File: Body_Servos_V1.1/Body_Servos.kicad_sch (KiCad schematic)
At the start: 30 parts, among them J1 USB_B_Micro, J12 SERIAL_FU, J2 AUX3, J3 AUX1, J4 AUX2, J5 12OUT, J6 12VOUT, J7 5V OUT, J8 5V Out 2, SW1 SW_Push, U1 ESP32-WROOM-32D_16MB_, U2 CJ2301_S1, U3 ME6211C33M5G, U4 CH340C, U5 UMH3N, U6 D36V50F5-STEPDOWN, U7 PCA9685

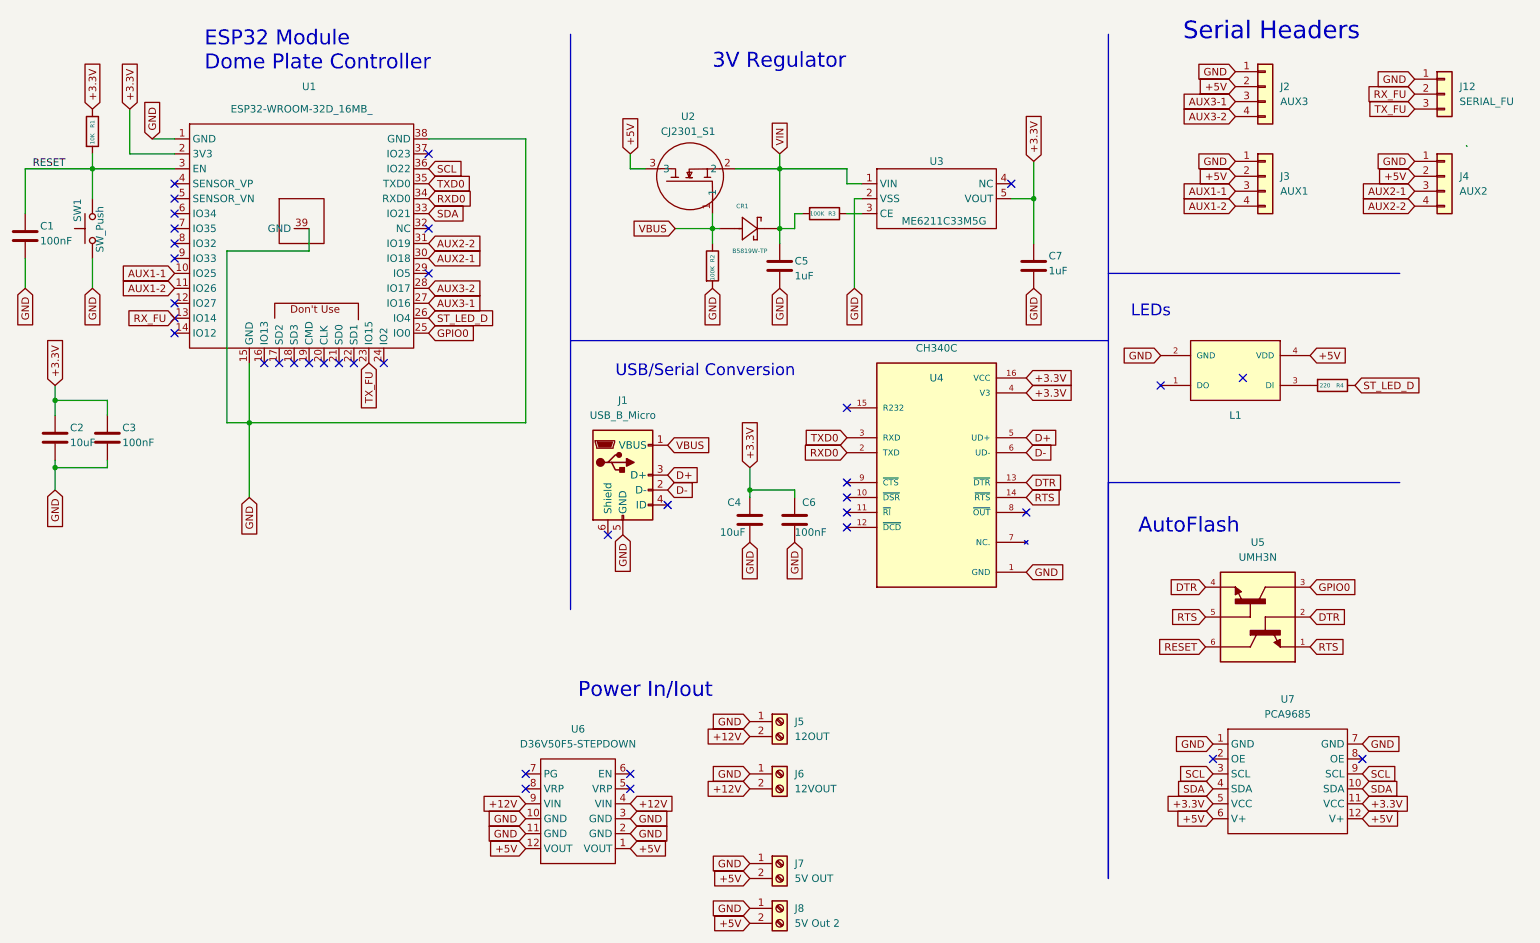
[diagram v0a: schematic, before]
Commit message: Updated C3P0 Controller
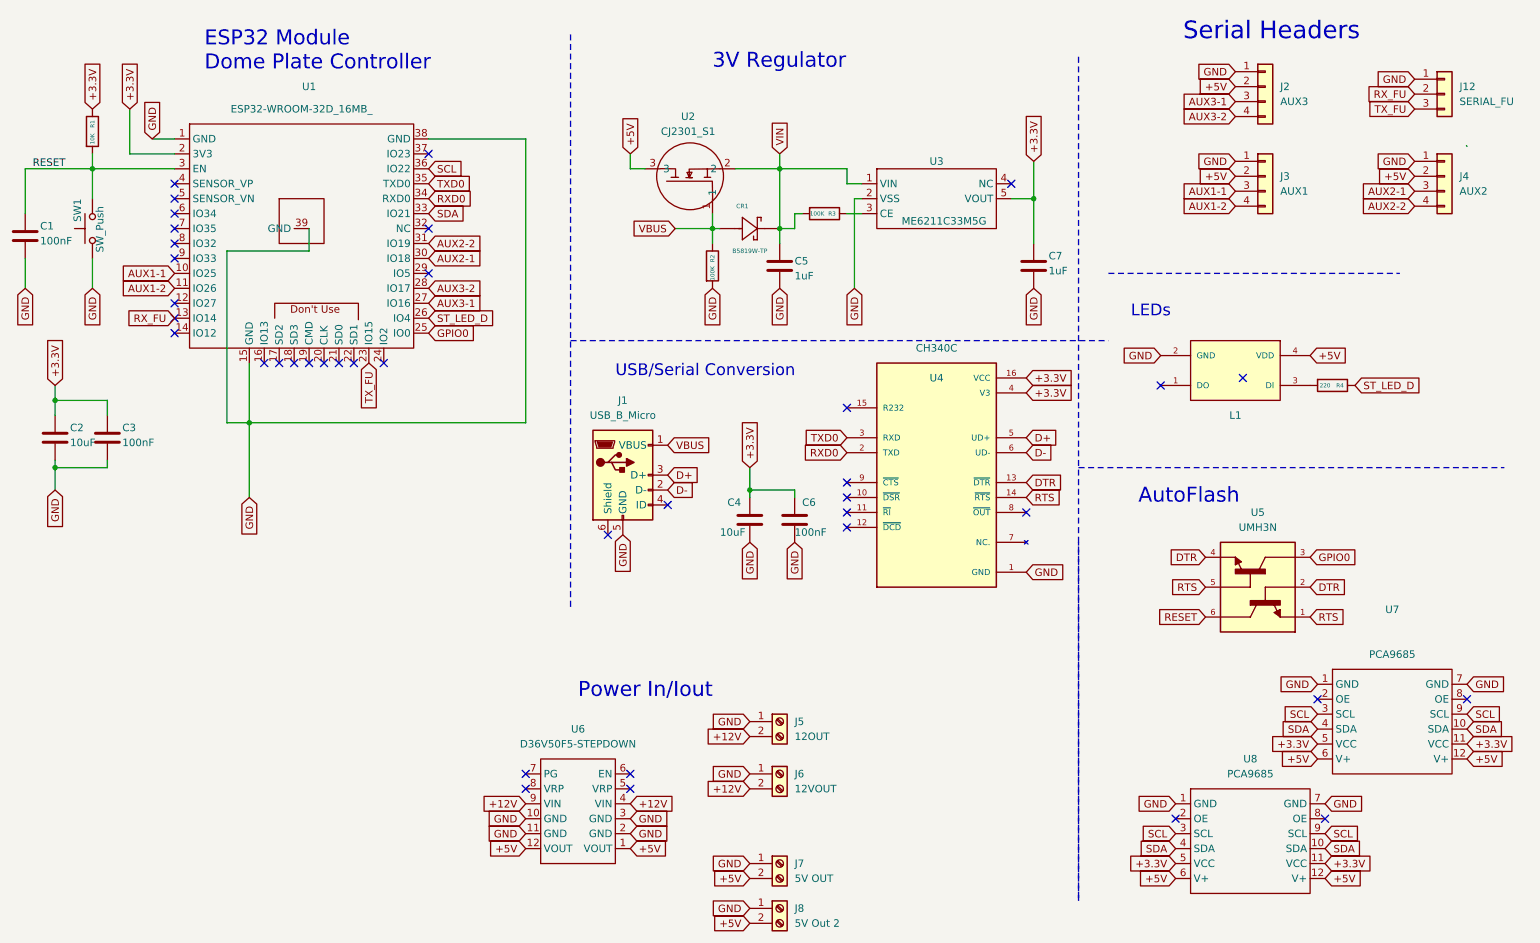
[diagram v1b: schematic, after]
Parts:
- added U8: PCA9685, 01-Custom:PCA9685, symbol Custom:PCA9685
- CR1: footprint Custom:SOD3716X135N -> 01-Custom:SOD3716X135N
- J2, J3, J4: footprint Custom:470531000 -> 01-Custom:470531000
- L1: footprint WS2812B-2020 -> 01-Custom:WS2812B-2020
- SW1: footprint Custom:TS-1101S-B-B-B-W-A -> 01-Custom:TS-1101S-B-B-B-W-A
- U4: footprint Custom:SOIC127P600X180-16N -> 01-Custom:SOIC127P600X180-16N
- U5: footprint Custom:UMT6 -> 01-Custom:UMT6
- U6: footprint Pololu:D36V50F5-STEPDOWN -> 01-Custom:D36V50F5-STEPDOWN
- U7: footprint Custom:PCA9685 -> 01-Custom:PCA9685
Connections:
- net +3.3V: now also U8.11 (VCC), U8.5 (VCC)
- net +5V: now also U8.12 (V+), U8.6 (V+)
- net GND: now also U8.1 (GND), U8.7 (GND)
- net SCL: now also U8.3 (SCL), U8.9 (SCL)
- net SDA: now also U8.10 (SDA), U8.4 (SDA)
- no-connect marks 37 -> 39
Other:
- moved on the sheet: U5, U7
